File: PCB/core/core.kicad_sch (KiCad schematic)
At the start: 2 parts, among them U1 MCU_Seeed_XIAO_ESP32-C3

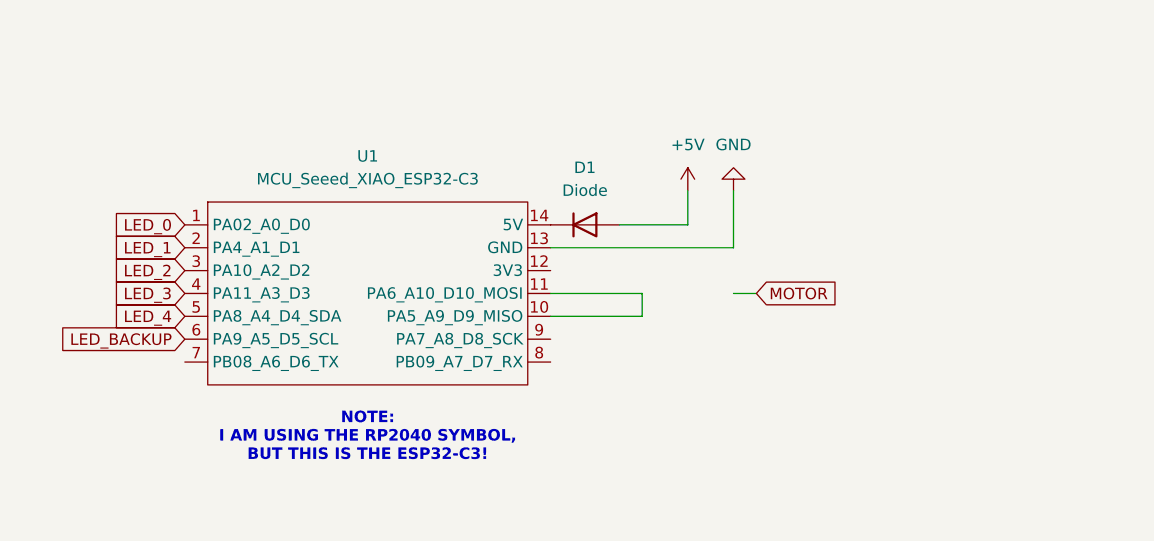
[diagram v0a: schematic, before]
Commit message: core PCB!!!
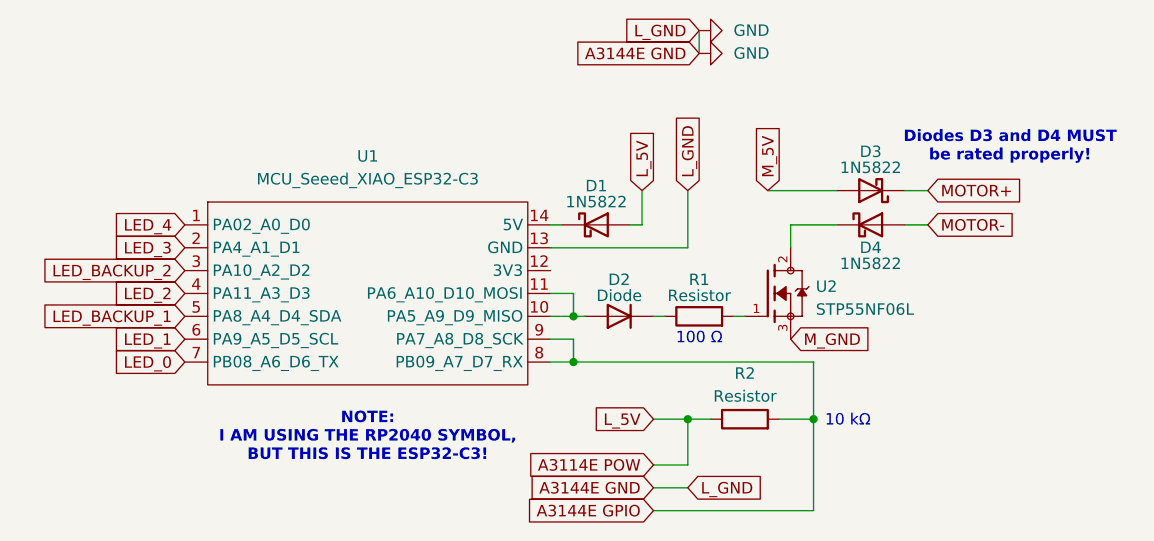
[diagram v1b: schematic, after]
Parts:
- removed D1: Diode, symbol ScottoKeebs:Placeholder_Diode
- added D1, D3, D4: 1N5822, Diode_THT:D_DO-201AD_P15.24mm_Horizontal, symbol Diode:1N5822
- added D2: Diode, ScottoKeebs_Components:Diode_DO-35, symbol ScottoKeebs:Placeholder_Diode
- added R1: Resistor, Resistor_THT:R_Axial_DIN0411_L9.9mm_D3.6mm_P20.32mm_Horizontal, symbol ScottoKeebs:Placeholder_Resistor
- added R2: Resistor, Resistor_THT:R_Axial_DIN0411_L9.9mm_D3.6mm_P15.24mm_Horizontal, symbol ScottoKeebs:Placeholder_Resistor
- added U2: STP55NF06L, STP55NF06L:TO254P1040X460X1935-3, symbol STP55NF06L:STP55NF06L
- U1: footprint (none) -> ScottoKeebs_MCU:Seeed_XIAO_RP2040
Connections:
- net LED_BACKUP is gone; now on net LED_1: U1.6 (PA9_A5_D5_SCL)
- net LED_0: now also U1.7 (PB08_A6_D6_TX); no longer U1.1 (PA02_A0_D0)
- net LED_1: no longer U1.2 (PA4_A1_D1)
- net LED_2: now also U1.4 (PA11_A3_D3); no longer U1.3 (PA10_A2_D2)
- net LED_3: now also U1.2 (PA4_A1_D1); no longer U1.4 (PA11_A3_D3)
- net LED_4: now also U1.1 (PA02_A0_D0); no longer U1.5 (PA8_A4_D4_SDA)
- net at U1.14 (5V): now also D1.1 (K)
- net at U1.10 (PA5_A9_D9_MISO), U1.11 (PA6_A10_D10_MOSI): now also D2.2 (A)
- net A3144E GPIO: now reaches U1.8 (PB09_A7_D7_RX)
- net A3144E GPIO: now also U1.9 (PA7_A8_D8_SCK), R2.2
- new net: D2.1 (K), R1.1
- new net: R1.2, U2.1
- new net: D4.1 (K), U2.2
- new net A3114E POW: D1.2 (A), R2.1
- new net LED_BACKUP_1: U1.5 (PA8_A4_D4_SDA)
- new net LED_BACKUP_2: U1.3 (PA10_A2_D2)
- new net MOTOR+: D3.1 (K)
- new net MOTOR-: D4.2 (A)
- new net M_5V: D3.2 (A)
- new net M_GND: U2.3
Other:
- note added: "10 kΩ"
- note added: "100 Ω"
- note added: "Diodes D3 and D4 MUST be rated properly!"
